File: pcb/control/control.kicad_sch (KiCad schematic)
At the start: 40 parts, among them J1 Barrel_Jack_MountingPin, J2 1729092, SW1 OS102011MS2QN1, SW2 OS102011MS2QN1, U1 PicoW, U2 SN65HVD230DR, U3 FDN340P, U4 DMG2305UX-7

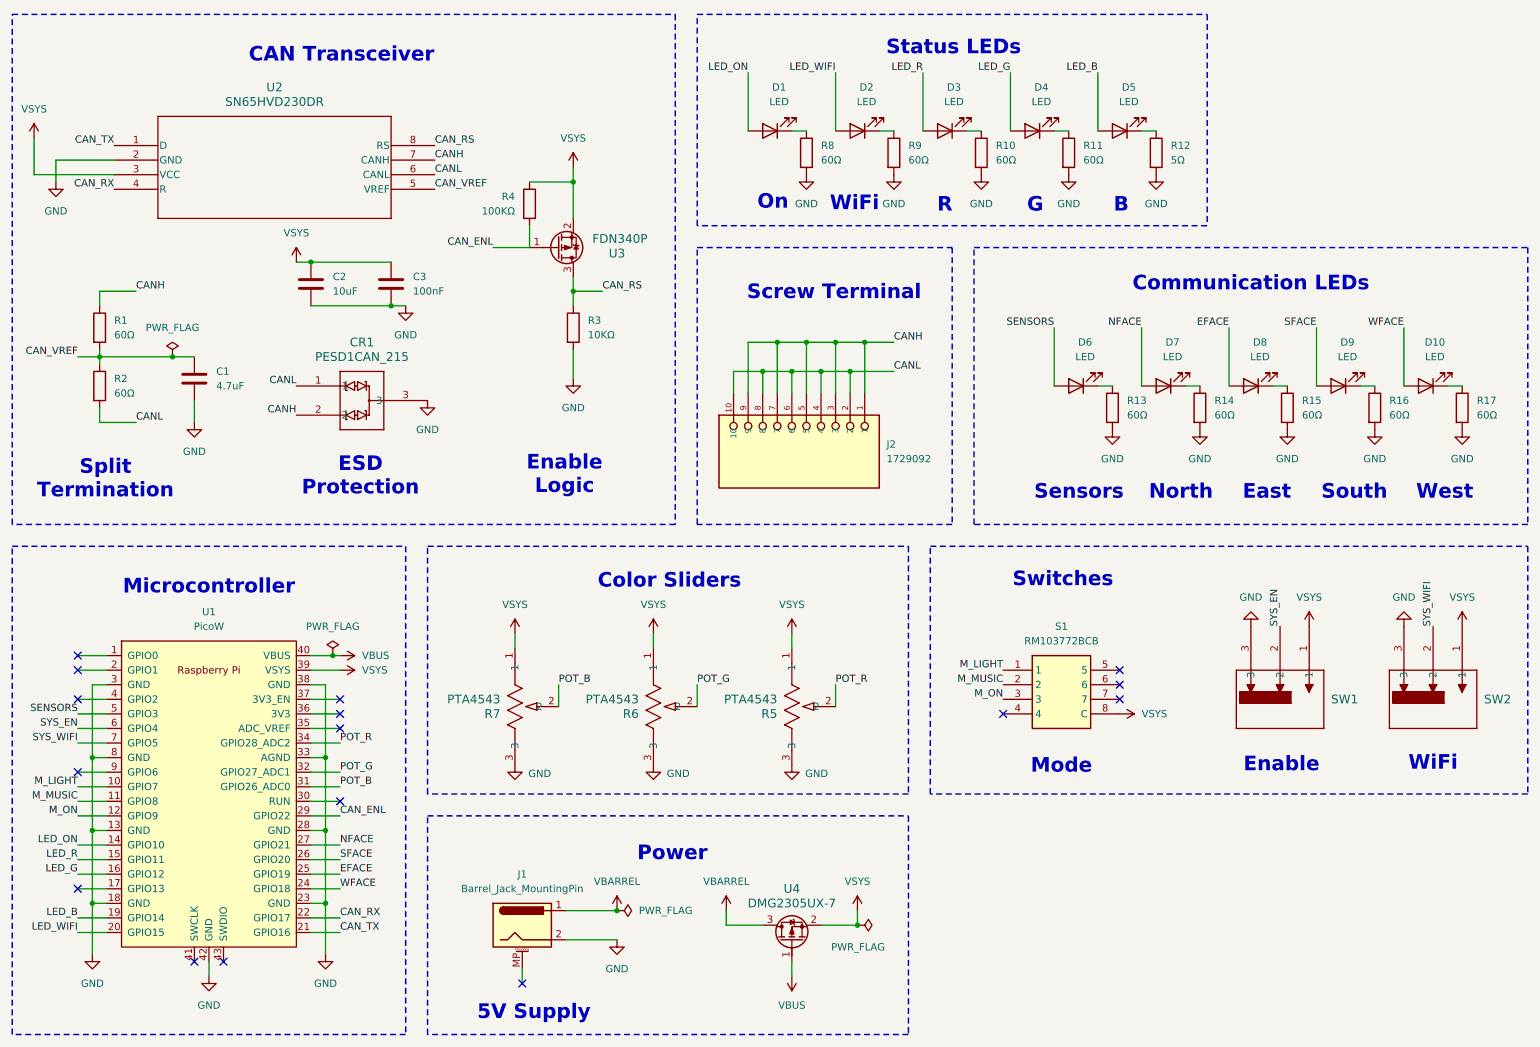
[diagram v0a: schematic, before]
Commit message: PCBs hopefully done
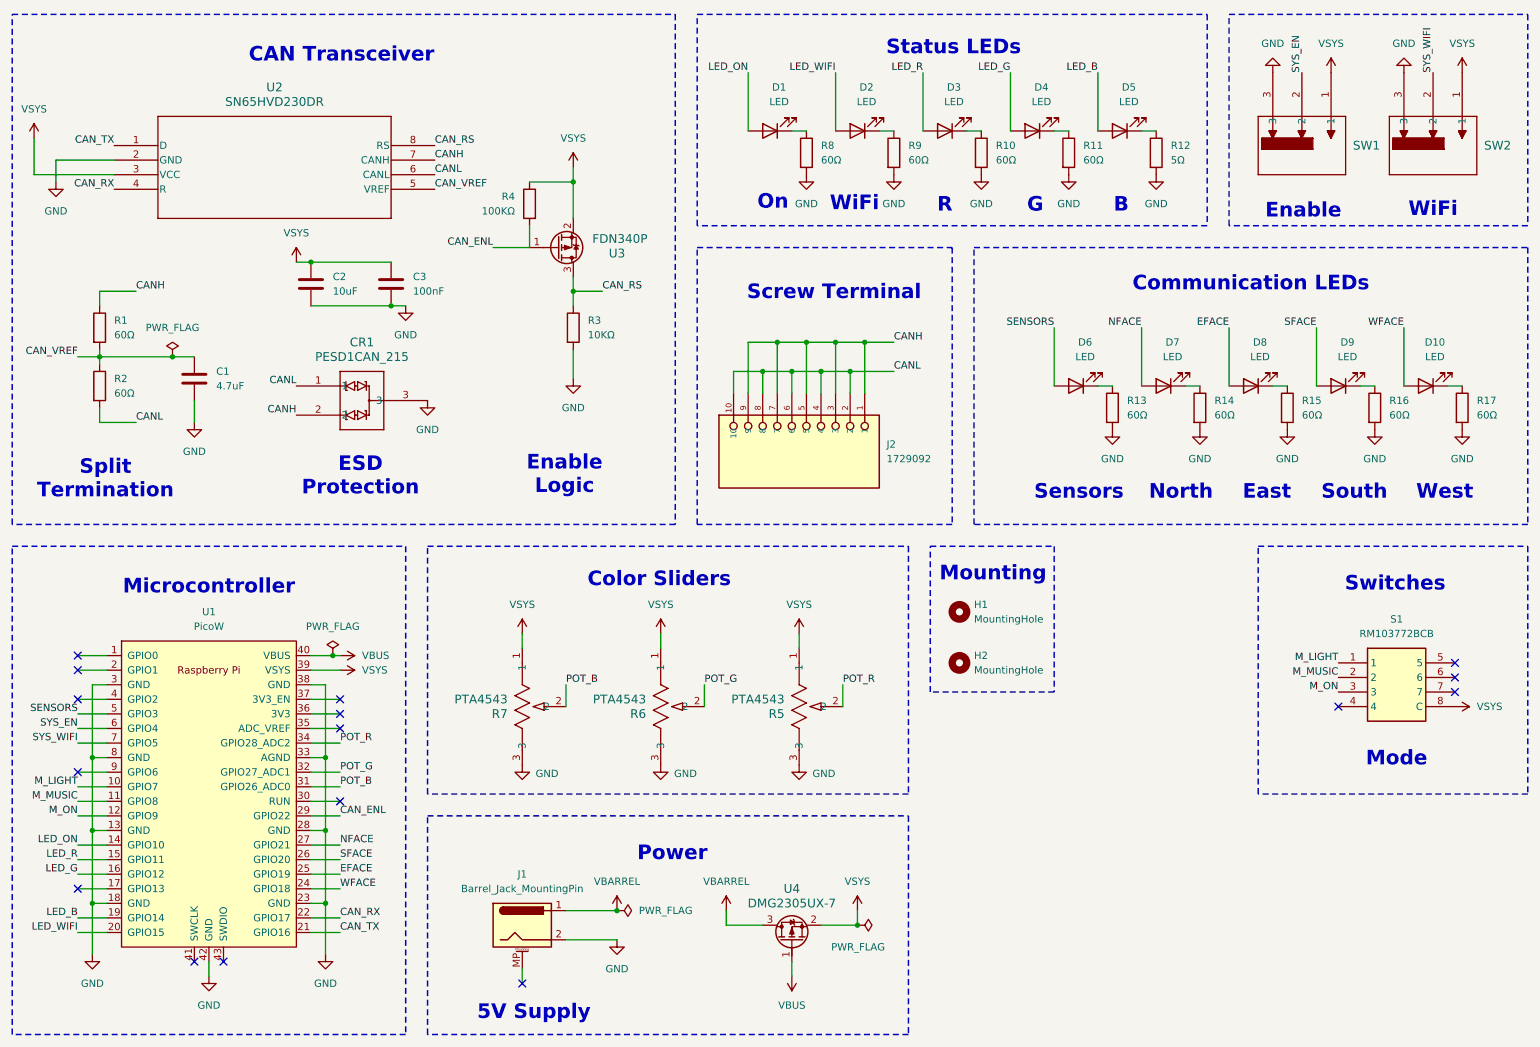
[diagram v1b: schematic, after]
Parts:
- added H1, H2: MountingHole, MountingHole:MountingHole_3.2mm_M3_DIN965_Pad, symbol Mechanical:MountingHole
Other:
- note added: "Mounting"
- moved on the sheet: R5, R6, R7, S1, SW1, SW2
